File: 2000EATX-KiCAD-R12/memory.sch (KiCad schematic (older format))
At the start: 30 parts, among them U500 KICKSTART, U501 74HCT00, U502 CY74FCT821T, U503 CY62157, U504 CY74FCT821T, U540 74AHCT244, U541 74AHCT244

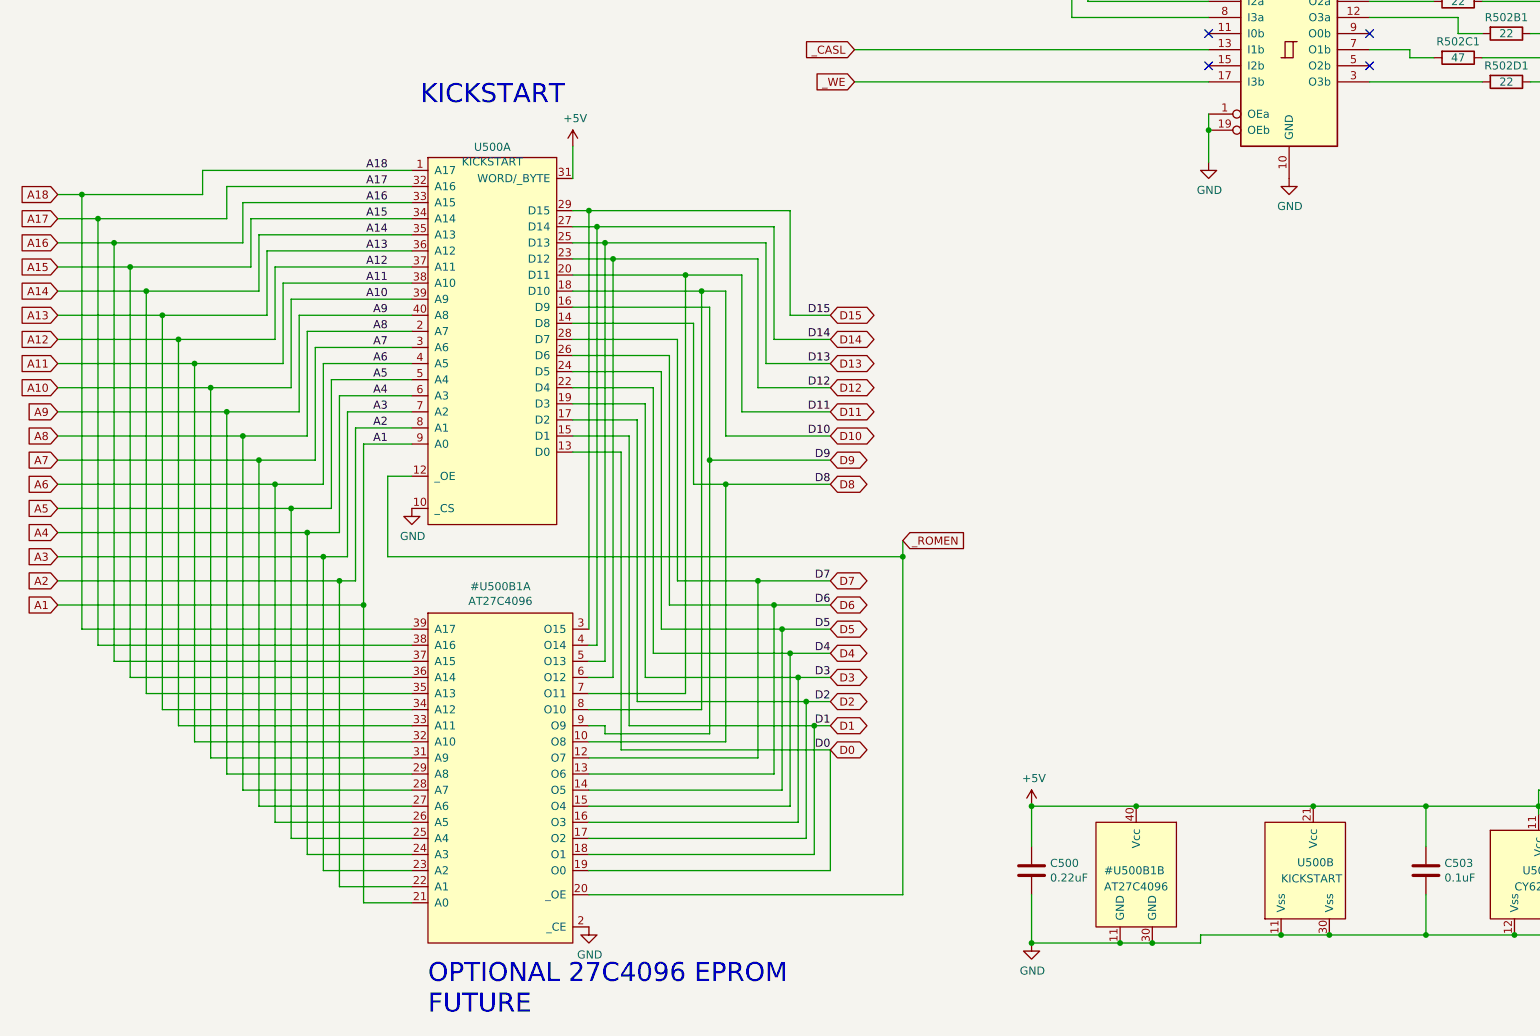
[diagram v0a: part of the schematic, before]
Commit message: Add files via upload
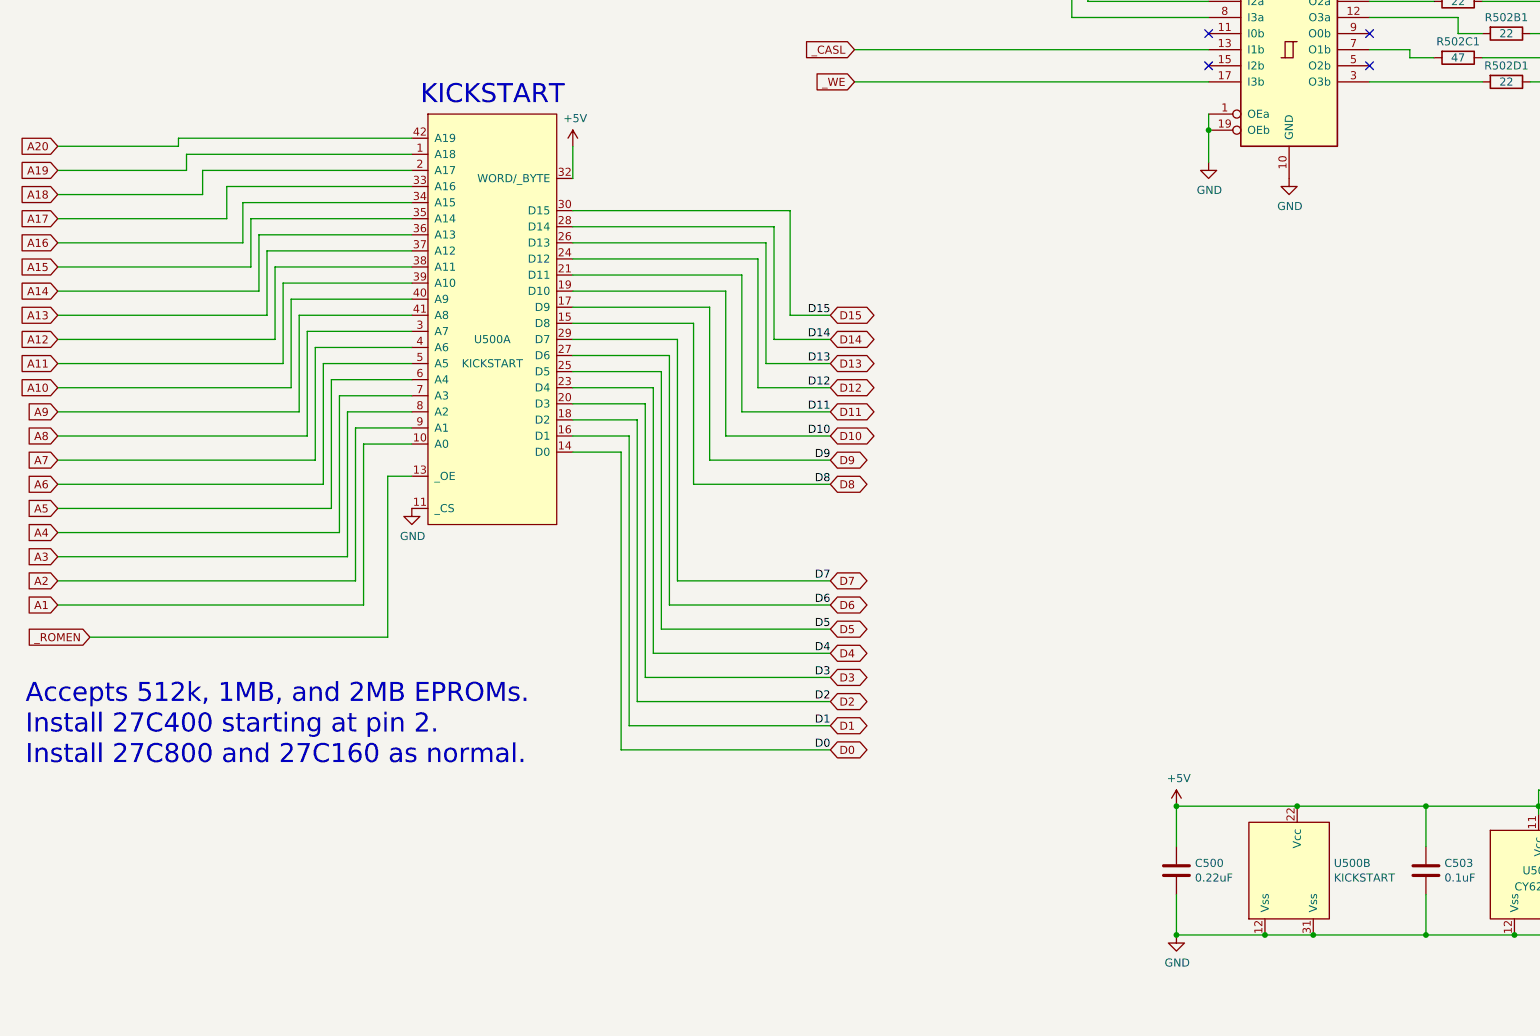
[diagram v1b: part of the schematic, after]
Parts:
- removed U500: KICKSTART, Package_DIP:DIP-40_W15.24mm, symbol Amiga-Library:27C400
- added U500: KICKSTART, Package_DIP:DIP-42_W15.24mm, symbol Amiga-Library:Kickstart
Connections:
- net +5V: now also U500.22 (Vcc), U500.32 (WORD/_BYTE)
- net A1: now also U500.10 (A0)
- net A10: now also U500.40 (A9)
- net A11: now also U500.39 (A10)
- net A12: now also U500.38 (A11)
- net A13: now also U500.37 (A12)
- net A14: now also U500.36 (A13)
- net A15: now also U500.35 (A14)
- net A16: now also U500.34 (A15)
- net A17: now also U500.33 (A16)
- net A18: now also U500.2 (A17)
- net A2: now also U500.9 (A1)
- net A3: now also U500.8 (A2)
- net A4: now also U500.7 (A3)
- net A5: now also U500.6 (A4)
- net A6: now also U500.5 (A5)
- net A7: now also U500.4 (A6)
- net A8: now also U500.3 (A7)
- net A9: now also U500.41 (A8)
- net D0: now also U500.14 (D0)
- net D1: now also U500.16 (D1)
- net D10: now also U500.19 (D10)
- net D11: now also U500.21 (D11)
- net D12: now also U500.24 (D12)
- net D13: now also U500.26 (D13)
- net D14: now also U500.28 (D14)
- net D15: now also U500.30 (D15)
- net D2: now also U500.18 (D2)
- net D3: now also U500.20 (D3)
- net D4: now also U500.23 (D4)
- net D5: now also U500.25 (D5)
- net D6: now also U500.27 (D6)
- net D7: now also U500.29 (D7)
- net D8: now also U500.15 (D8)
- net D9: now also U500.17 (D9)
- net GND: now also U500.11 (_CS), U500.12 (Vss), U500.31 (Vss)
- net _ROMEN: now also U500.13 (_OE)
- new net A19: U500.1 (A18)
- new net A20: U500.42 (A19)
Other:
- note added: "Accepts 512k, 1MB, and 2MB EPROMs.\nInstall 27C400 starting at pin 2.\nInstall 27C800 and 27C160 as normal."
- note removed: "OPTIONAL 27C4096 EPROM\nFUTURE"
- moved on the sheet: C500
